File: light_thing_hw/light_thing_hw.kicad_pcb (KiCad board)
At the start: 2 copper layers, 42 x 42 mm, 50 parts, among them J1 CONNECTORS, J2 Li-Ion Battery, J3 ADDR_LED_PANEL_1_CONNECTORS, J4 ADDR_LED_PANEL_2_CONNECTORS, Q1 MMBF170, SW1 ST_USER_BUTTON1, SW2 ST_RESET_BUTTON, U1 BC832-V1, U2 LSM6DS3, U3 MCP73833T-FCI_MF, U4 LMR62421XMF, U5 LP38511MRX-ADJ_NOPB, U5A1 STM32L452RETx

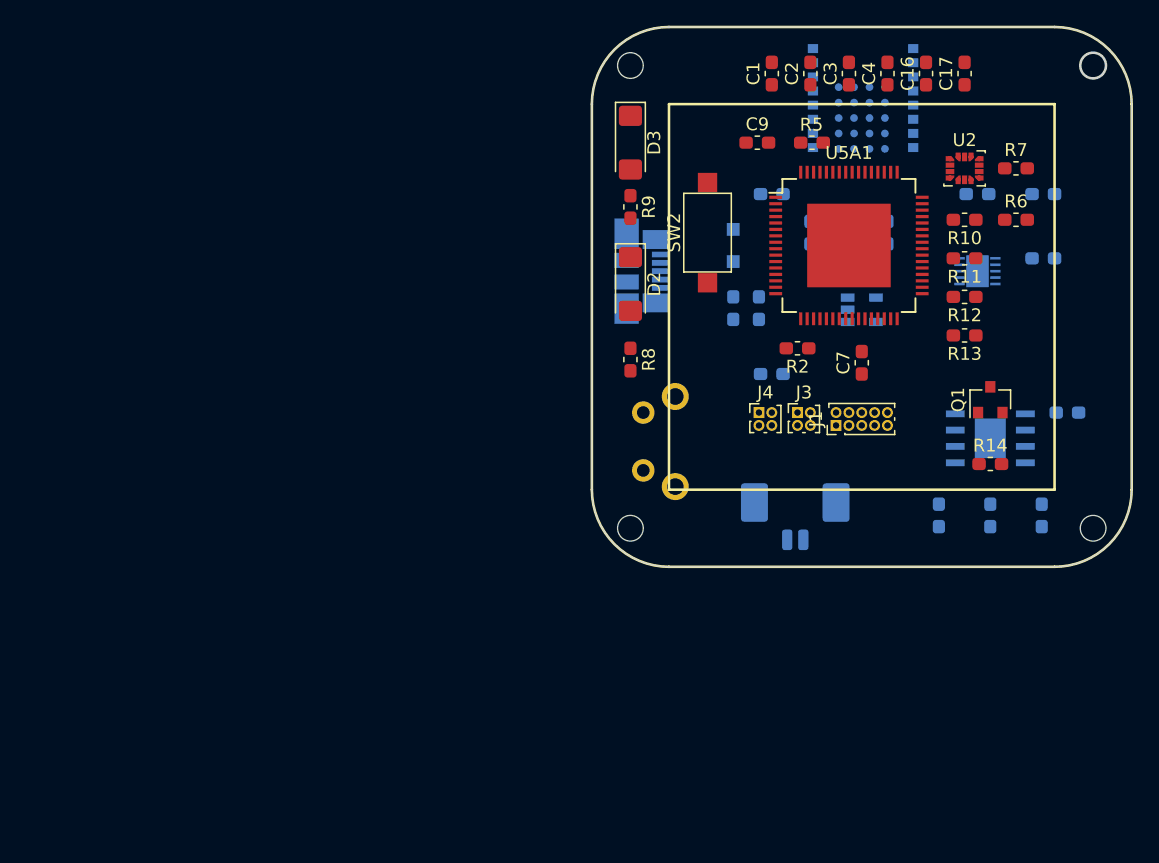
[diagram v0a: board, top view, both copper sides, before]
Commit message: made 5cm pcb. need to do routing etc.
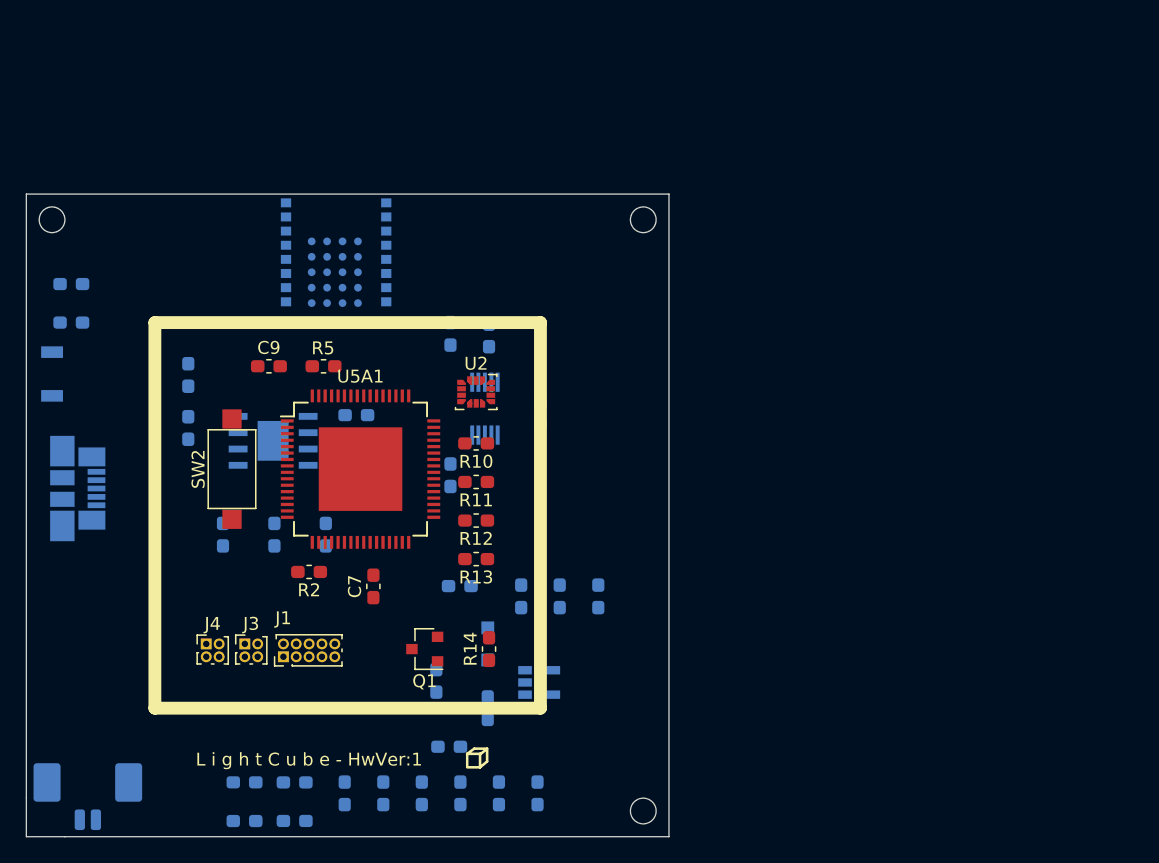
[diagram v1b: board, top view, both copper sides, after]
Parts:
- added C15: 2700pF, Capacitor_SMD:C_0603_1608Metric_Pad1.05x0.95mm_HandSolder, B.Cu at (119.6, 70.1)
- added C18: 10uF, Capacitor_SMD:C_0603_1608Metric_Pad1.05x0.95mm_HandSolder, B.Cu at (119.6, 74.2)
- added R17: 1k, Resistor_SMD:R_0603_1608Metric_Pad1.05x0.95mm_HandSolder, B.Cu at (147.0, 73.1)
- C1, C16, C17, C2, C3, C4, R8, R9: moved to B.Cu
- D2, D3: footprint LED_SMD:LED_1806_4516Metric_Pad1.57x1.80mm_HandSolder -> LED_SMD:LED_0603_1608Metric_Pad1.05x0.95mm_HandSolder; moved to B.Cu
- R1: value 800 -> 1k
- R15: value 3.5k -> 2k
- R16: value 3.5k -> 357
- R6: value R -> 4.7k; moved to B.Cu
- R7: value R -> 100; moved to B.Cu
- SW1: footprint Button_Switch_THT:SW_Tactile_SPST_Angled_PTS645Vx39-2LFS -> Button_Switch_SMD:SW_SPST_B3U-3000P
- U3: value MCP73833T-FCI_MF -> MCP73833T-FCI_UN; footprint footprints:MCP73833T-FCI&slash_MF -> footprints:MCP73833T-FCIUN-SMD
- moved R7 74.5 mm to (110.5, 66.0)
- moved C17 73.9 mm to (131.8, 102.6)
- moved R6 73.7 mm to (110.5, 63.0)
- moved C16 70.1 mm to (134.8, 102.6)
- moved C4 66.7 mm to (137.8, 102.6)
- moved C3 63.6 mm to (140.8, 102.6)
- moved C2 61.0 mm to (143.8, 102.6)
- moved J2 59.2 mm to (111.8, 102.3)
- moved C1 58.9 mm to (146.8, 102.6)
- moved D3 58.9 mm to (127.9, 104.8), turned to 180 degrees
- moved R9 56.4 mm to (124.0, 104.8), turned to 180 degrees
- moved U5 55.8 mm to (126.2, 75.2)
- moved R15 55.7 mm to (122.3, 82.5)
- moved R16 55.7 mm to (126.3, 82.5)
- moved C14 55.7 mm to (130.3, 82.5)
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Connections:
- C1 pad 2: +5V -> GND
- C10 pad 2: +5V -> GND
- C11 pad 2: +5V -> GND
- C14 pad 2: +5V -> GND
- C16 pad 2: +5V -> GND
- C17 pad 2: +5V -> GND
- C2 pad 2: +5V -> GND
- C3 pad 2: +5V -> GND
- C4 pad 2: +5V -> GND
- C5 pad 2: +5V -> GND
- C6 pad 2: +5V -> Net-(C6-Pad2)
- C7 pad 2: +5V -> GND
- C8 pad 1: +5V -> GND
- C9 pad 2: +5V -> GND
- D2 pad 1: +5V -> GND
- D3 pad 1: +5V -> GND
- J2 pad 1: +5V -> GND
- J3 pad 1: +5V -> GND
- J3 pad 4: +5V -> GND
- J4 pad 1: +5V -> GND
- J4 pad 4: +5V -> GND
- Q1 pad 2: +5V -> GND
- R1 pad 1: +5V -> VBUS
- R16 pad 1: +5V -> GND
- R4 pad 2: +5V -> GND
- R5 pad 2: +5V -> GND
- R6 pad 2: +5V -> GND
- R7 pad 1: +5V -> GND
- SW1 pad 1: +5V -> GND
- SW2 pad 1: +5V -> GND
- U1 pad P$1: +5V -> GND
- U2 pad 1: +5V -> GND
- U2 pad 2: +5V -> GND
- U2 pad 3: +5V -> GND
- U2 pad 6: +5V -> GND
- U2 pad 7: +5V -> GND
- U3 pad 10: +BATT -> Net-(C6-Pad2)
- U3 pad 3: Net-(U3-Pad3) -> CHARGER_STAT1
- U3 pad 4: Net-(U3-Pad4) -> CHARGER_STAT2
- U3 pad 5: +5V -> GND
- U3 pad 6: Net-(R1-Pad2) -> Net-(R17-Pad2)
- U3 pad 7: Net-(U3-Pad7) -> Net-(R1-Pad2)
- U3 pad 9: +BATT -> Net-(C6-Pad2)
- U4 pad 2: +5V -> GND
- U5 pad 5: +5V -> GND
- U5 pad 9: +5V -> GND
- U5A1 pad 12: +5V -> GND
- U5A1 pad 18: +5V -> GND
- U5A1 pad 30: Net-(U5A1-Pad30) -> I2C2_SDA
- U5A1 pad 31: +5V -> GND
- U5A1 pad 35: I2C2_SDA -> CHARGER_STAT1
- U5A1 pad 36: Net-(U5A1-Pad36) -> CHARGER_STAT2
- U5A1 pad 47: +5V -> GND
- U5A1 pad 63: +5V -> GND
- USB_MICRO_CONN1 pad 5: +5V -> GND
- USB_MICRO_CONN1 pad 6: Net-(USB_MICRO_CONN1-Pad6) -> GND
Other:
- board size 42 x 42 mm -> 50 x 50 mm
- board text added: "L i g h t C u b e - HwVer:1"
